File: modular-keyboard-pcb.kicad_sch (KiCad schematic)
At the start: 2 parts, among them J1 Conn_01x02, U1 nice_nano

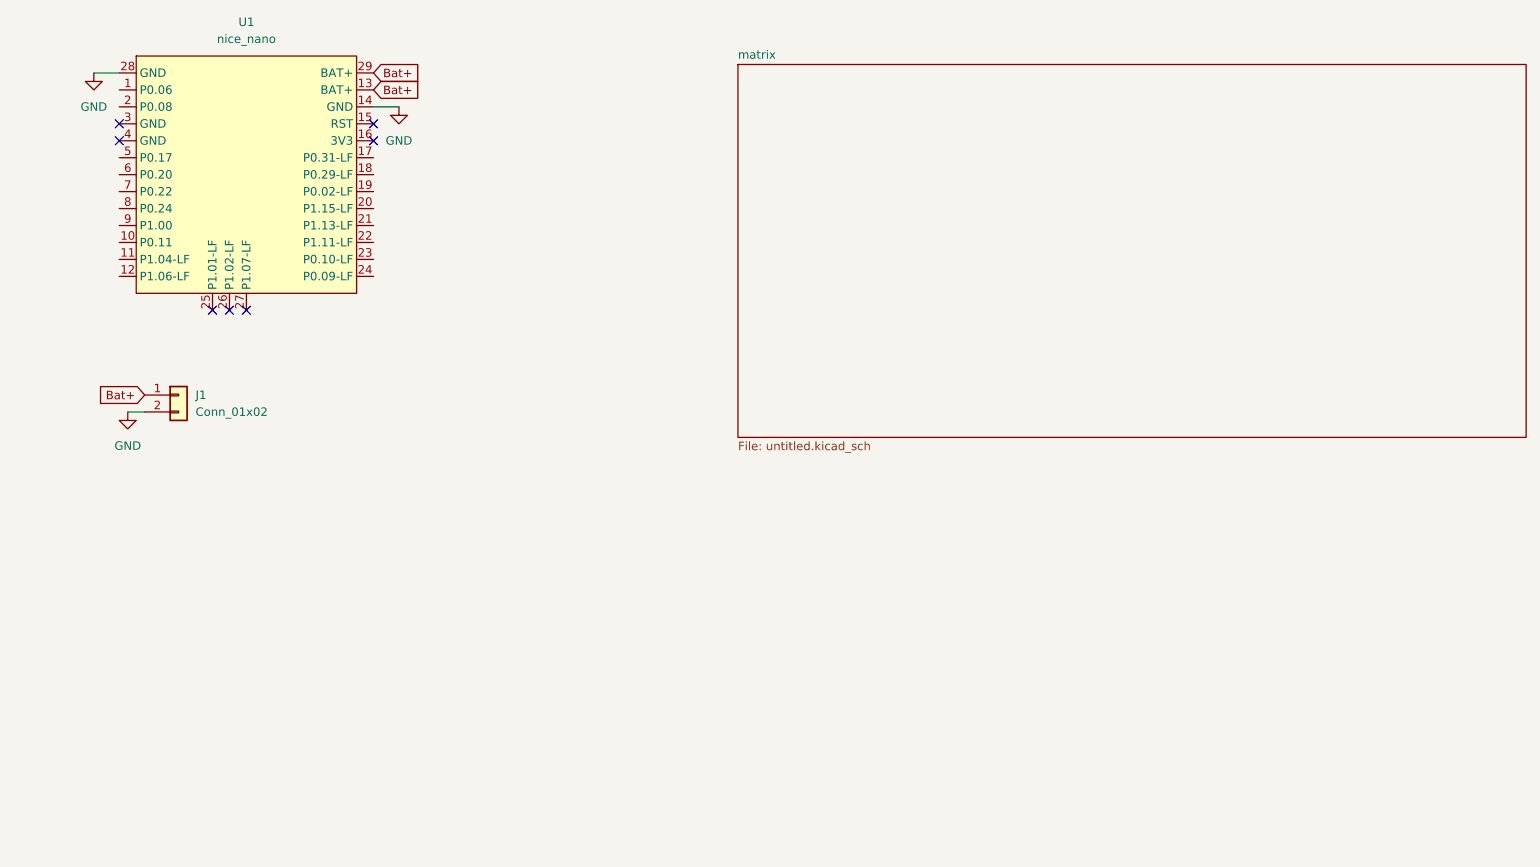
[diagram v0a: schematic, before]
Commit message: day 2 end
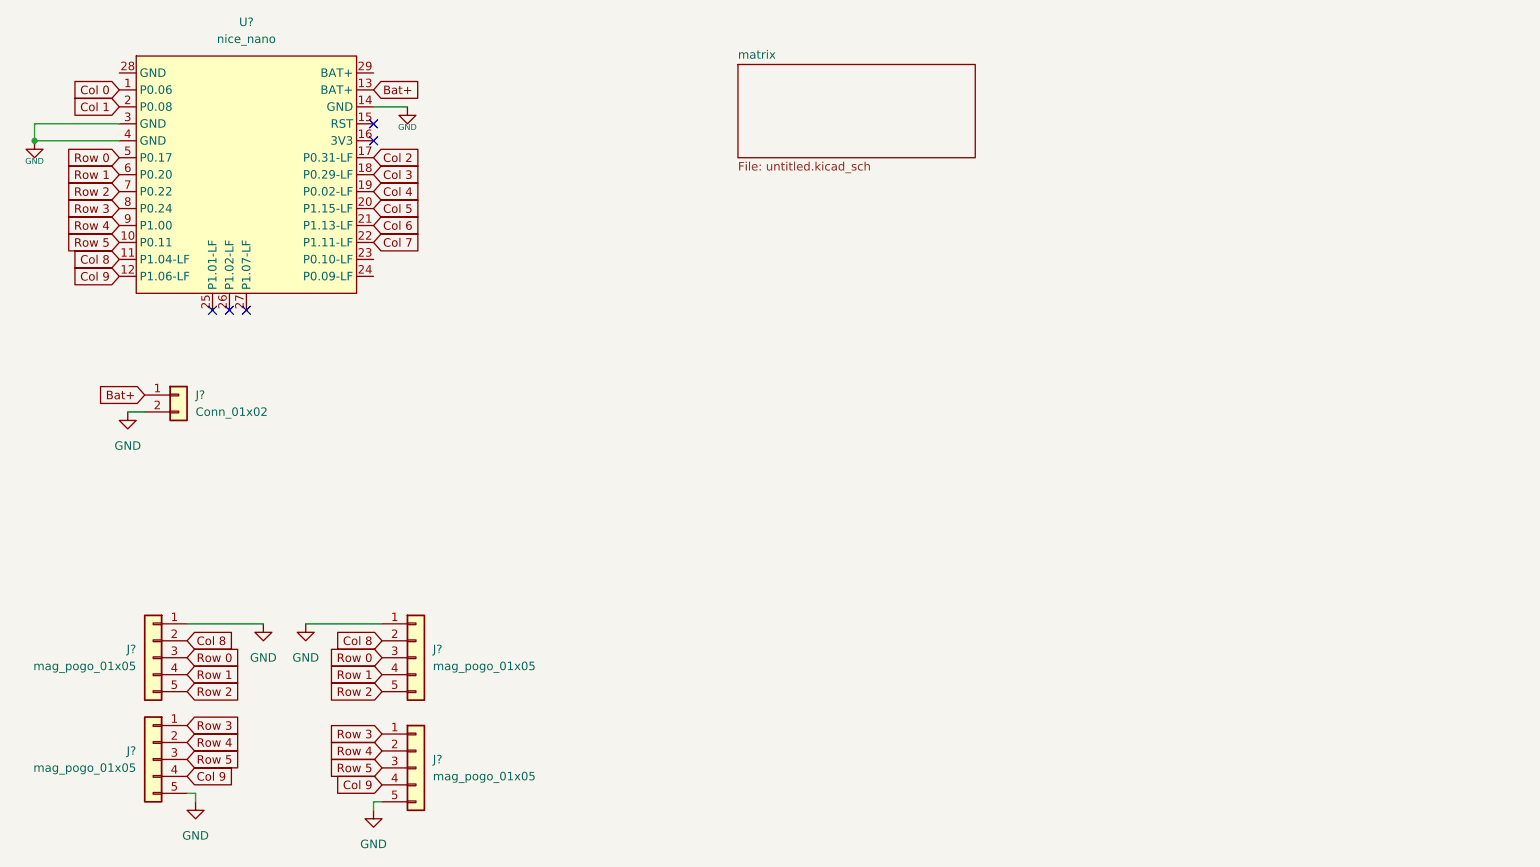
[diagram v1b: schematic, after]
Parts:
- added J? (x4): mag_pogo_01x05, symbol Connector_Generic:Conn_01x05
- renumbered J1 to J?, U1 to U?
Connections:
- net Bat+: no longer U?.29 (BAT+)
- net GND: now also U?.3 (GND), U?.4 (GND), J?.1 (Pin_1), J?.1 (Pin_1), J?.5 (Pin_5), J?.5 (Pin_5); no longer U?.28 (GND)
- net Col 0: now reaches U?.1 (P0.06)
- net Row 5: now reaches U?.10 (P0.11)
- net Row 5: now also J?.3 (Pin_3), J?.3 (Pin_3)
- net Col 8: now reaches U?.11 (P1.04-LF)
- net Col 8: now also J?.2 (Pin_2), J?.2 (Pin_2)
- net Col 9: now reaches U?.12 (P1.06-LF)
- net Col 9: now also J?.4 (Pin_4), J?.4 (Pin_4)
- net Col 2: now reaches U?.17 (P0.31-LF)
- net Col 3: now reaches U?.18 (P0.29-LF)
- net Col 4: now reaches U?.19 (P0.02-LF)
- net Col 1: now reaches U?.2 (P0.08)
- net Col 5: now reaches U?.20 (P1.15-LF)
- net Col 6: now reaches U?.21 (P1.13-LF)
- net Col 7: now reaches U?.22 (P1.11-LF)
- net Row 0: now reaches U?.5 (P0.17)
- net Row 0: now also J?.3 (Pin_3), J?.3 (Pin_3)
- net Row 1: now reaches U?.6 (P0.20)
- net Row 1: now also J?.4 (Pin_4), J?.4 (Pin_4)
- net Row 2: now reaches U?.7 (P0.22)
- net Row 2: now also J?.5 (Pin_5), J?.5 (Pin_5)
- net Row 3: now reaches U?.8 (P0.24)
- net Row 3: now also J?.1 (Pin_1), J?.1 (Pin_1)
- net Row 4: now reaches U?.9 (P1.00)
- net Row 4: now also J?.2 (Pin_2), J?.2 (Pin_2)
- no-connect marks 7 -> 5
